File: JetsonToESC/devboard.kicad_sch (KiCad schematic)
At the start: 6 parts, among them U1 ESP32-C3_SUPERMINI_TH

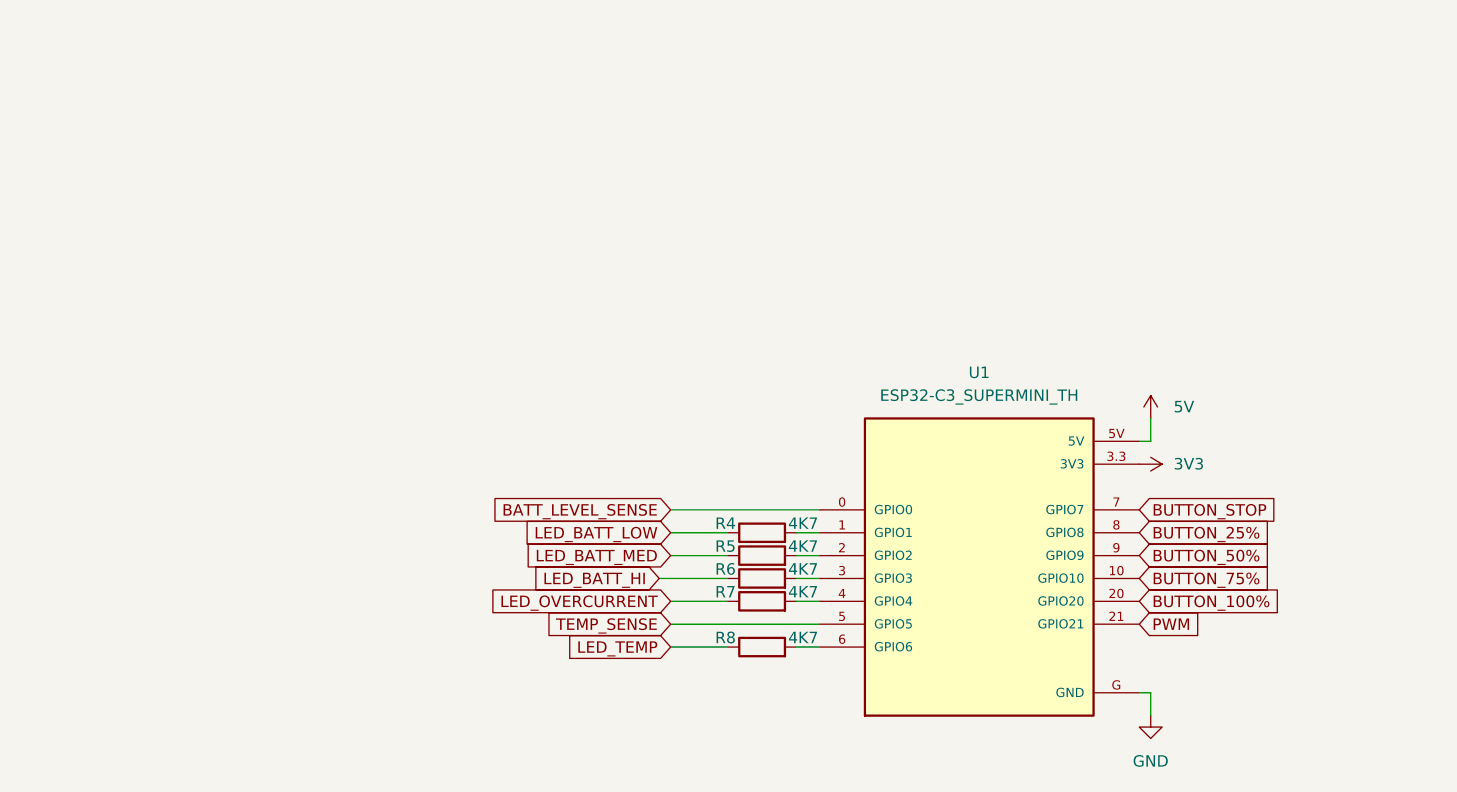
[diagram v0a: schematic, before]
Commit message: Start On this Branch
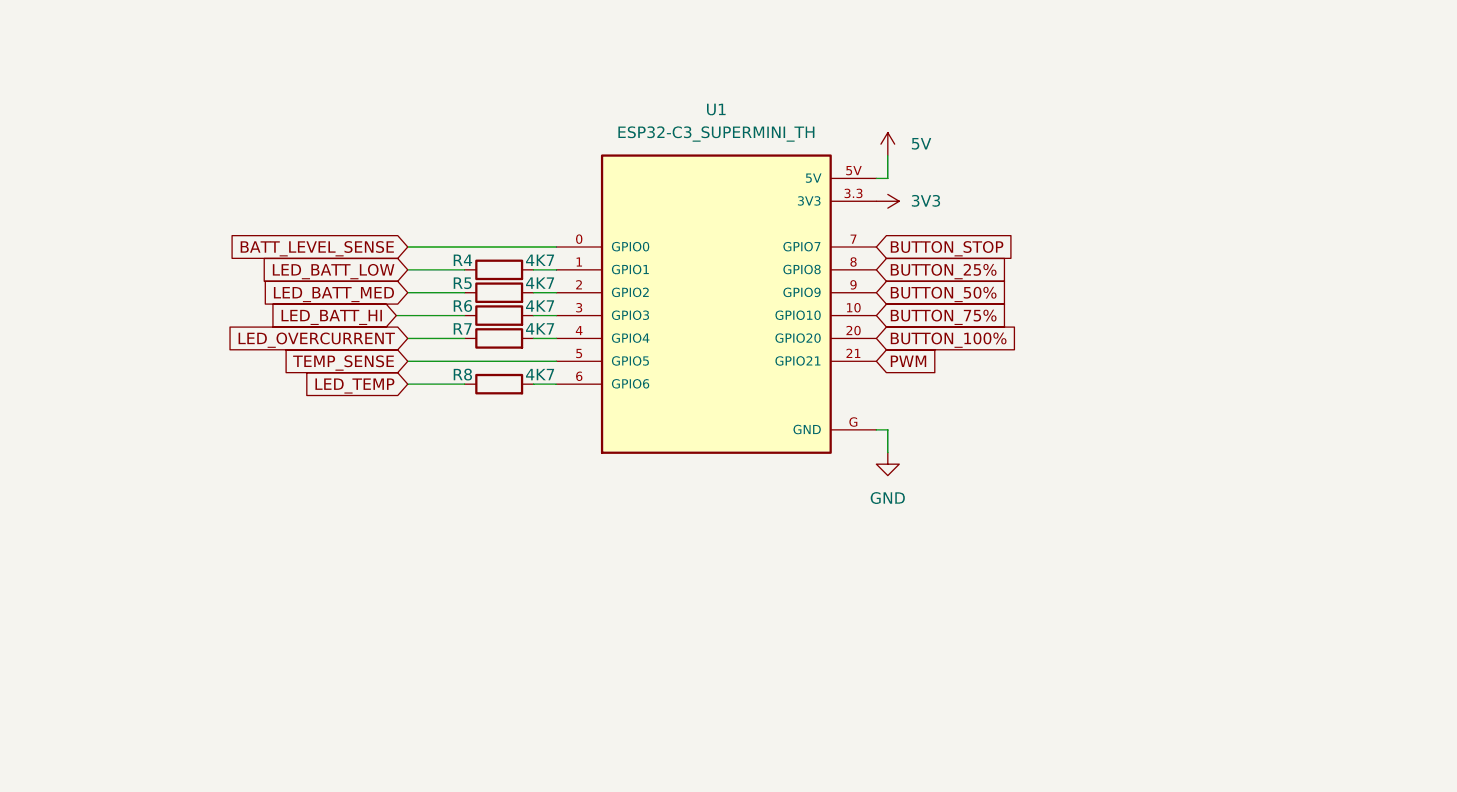
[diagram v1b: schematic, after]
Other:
- moved on the sheet: R4, R5, R6, R7, R8, U1

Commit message: updated too
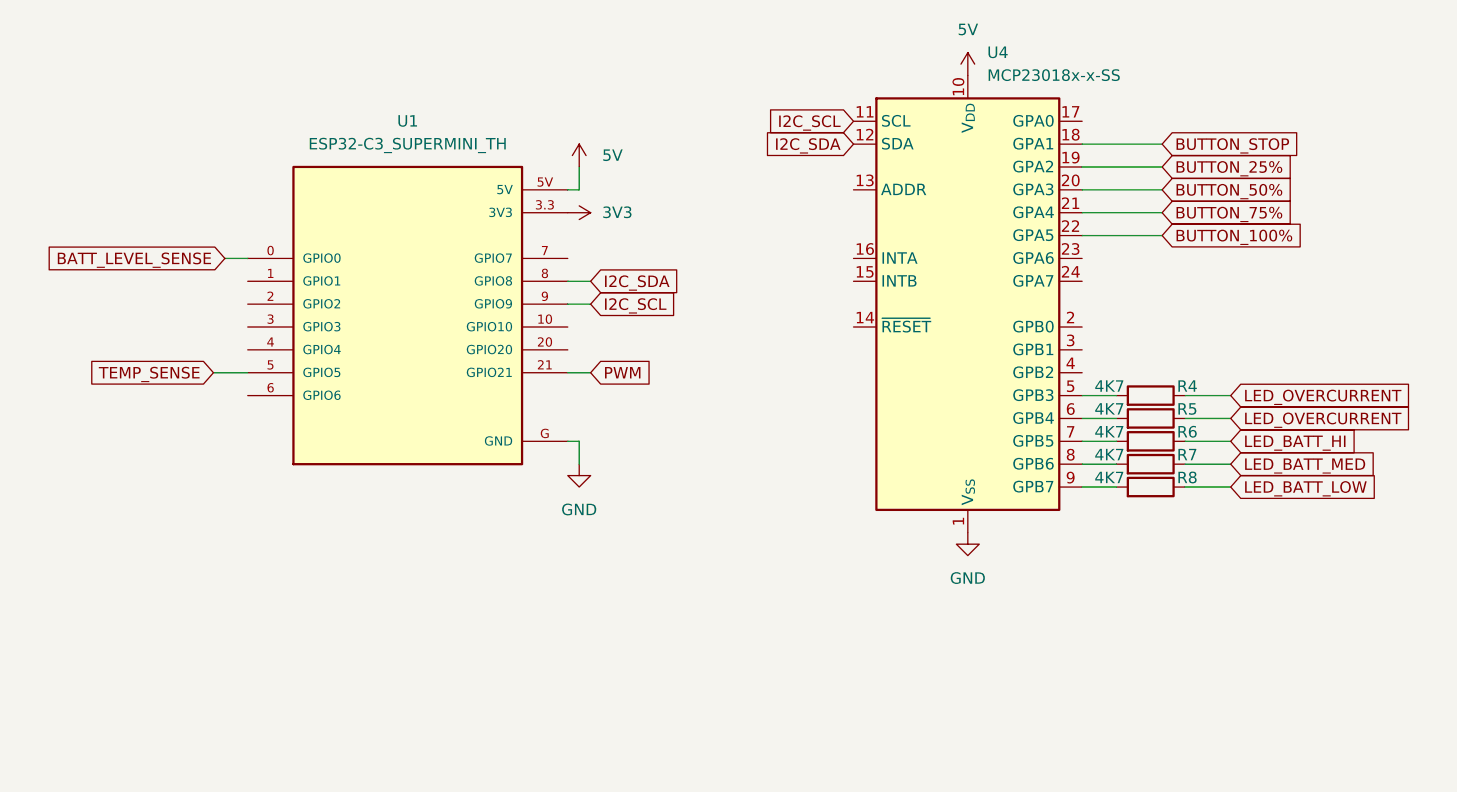
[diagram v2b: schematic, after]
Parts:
- added U4: MCP23018x-x-SS, Package_SO:SSOP-24_5.3x8.2mm_P0.65mm, symbol Interface_Expansion:MCP23018x-x-SS
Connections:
- net LED_TEMP is gone; now on net LED_BATT_LOW: R8.1
- net 5V: now also U4.10 (V_{DD})
- net BUTTON_100%: now also U4.22 (GPA5); no longer U1.20 (GPIO20)
- net BUTTON_25%: now also U4.19 (GPA2); no longer U1.8 (GPIO8)
- net BUTTON_50%: now also U4.20 (GPA3); no longer U1.9 (GPIO9)
- net BUTTON_75%: now also U4.21 (GPA4); no longer U1.10 (GPIO10)
- net BUTTON_STOP: now also U4.18 (GPA1); no longer U1.7 (GPIO7)
- net GND: now also U4.1 (V_{SS})
- net LED_BATT_LOW: no longer R4.1
- net LED_BATT_MED: now also R7.1; no longer R5.1
- net LED_OVERCURRENT: now also R4.1, R5.1; no longer R7.1
- net at R7.2: now also U4.8 (GPB6); no longer U1.4 (GPIO4)
- net at R6.2: now also U4.7 (GPB5); no longer U1.3 (GPIO3)
- net at R4.2: now also U4.5 (GPB3); no longer U1.1 (GPIO1)
- net at R5.2: now also U4.6 (GPB4); no longer U1.2 (GPIO2)
- net at R8.2: now also U4.9 (GPB7); no longer U1.6 (GPIO6)
- new net I2C_SCL: U1.9 (GPIO9), U4.11 (SCL)
- new net I2C_SDA: U1.8 (GPIO8), U4.12 (SDA)
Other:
- moved on the sheet: R4, R5, R6, R7, R8, U1
